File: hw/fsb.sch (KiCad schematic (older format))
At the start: 8 parts, among them J101 AMPSEAL_8_POS_VERT_WHITE_SEAL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, J102 AMPSEAL_23_POS_VERT_WHITE_SEA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

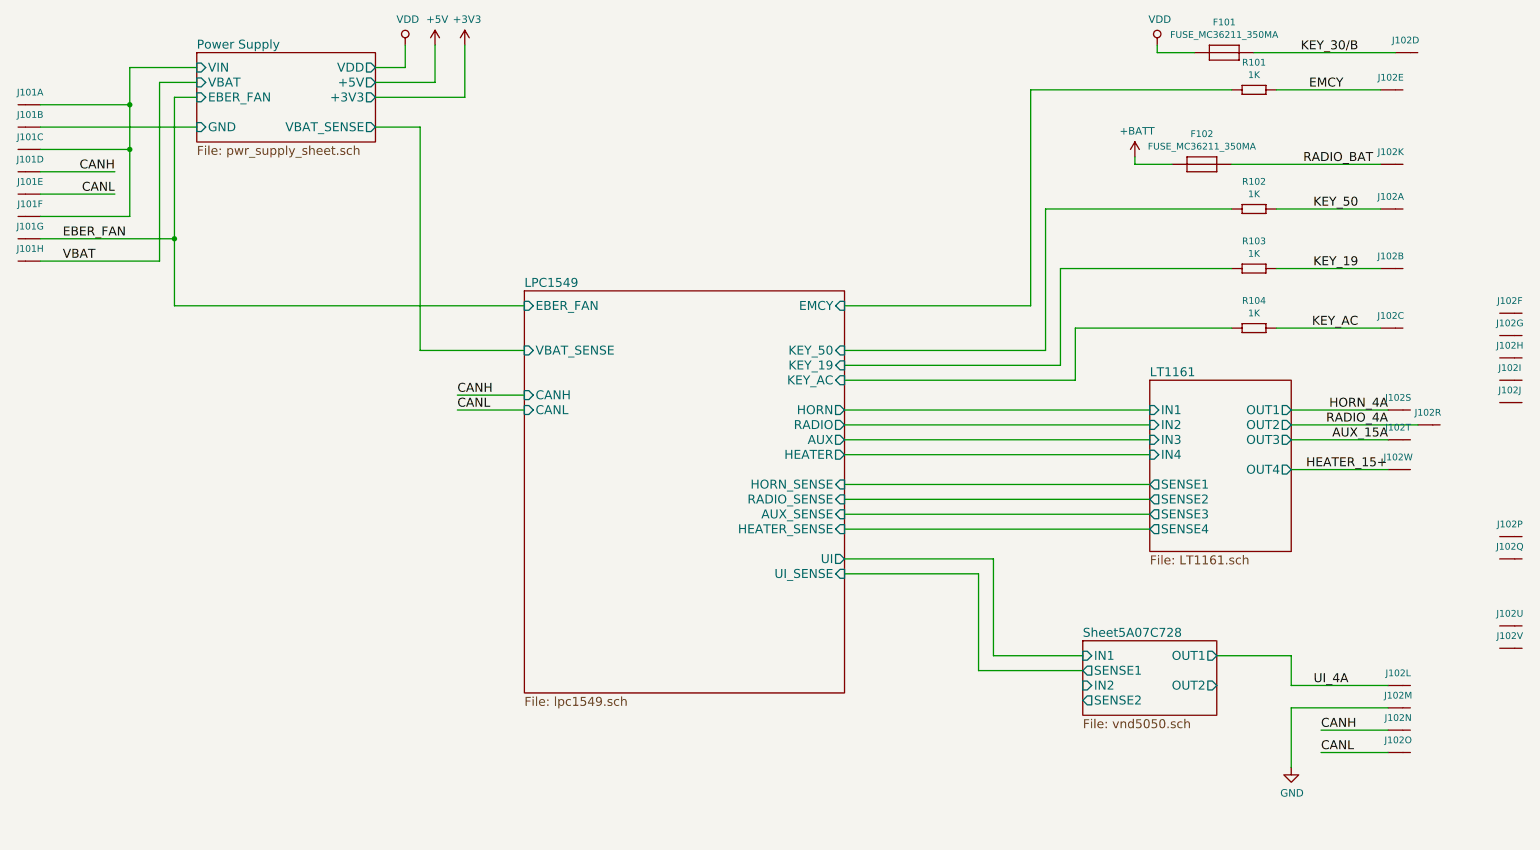
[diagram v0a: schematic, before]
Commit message: hw 2.1.0 created, not yet ordered
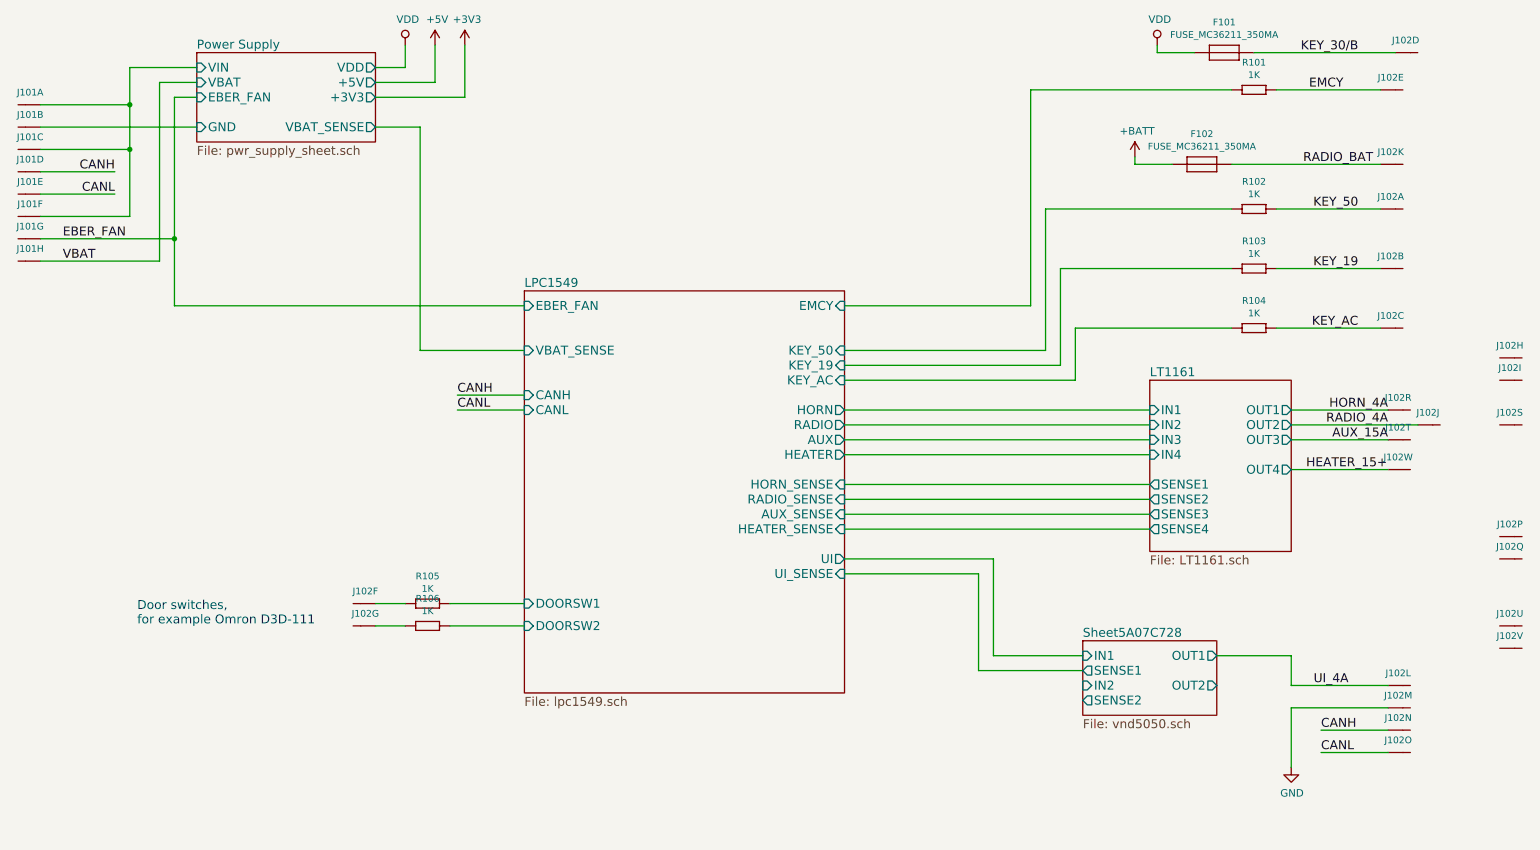
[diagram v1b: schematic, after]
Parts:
- added R105, R106: 1K, yageo:0603, symbol 1K
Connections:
- net HORN_4A: now also J102.P$18 (S); no longer J102.P$19 (S)
- net RADIO_4A: now also J102.P$10 (S); no longer J102.P$18 (S)
- net at J102.P$6 (S): now also R105.2 (R2)
- net at J102.P$7 (S): now also R106.2 (R2)
- new net LPC1549/DOORSW1: R105.1 (R1)
- new net LPC1549/DOORSW2: R106.1 (R1)
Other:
- note added: "Door switches,\nfor example Omron D3D-111"
- moved on the sheet: J102F, J102G, J102J, J102R, J102S
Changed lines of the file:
@@
 F18 "UI" O R 6400 4600 60
 F19 "UI_SENSE" I R 6400 4700 60
+F20 "DOORSW1" I L 4250 4900 60
+F21 "DOORSW2" I L 4250 5050 60
 $EndSheet
 $Comp
@@
 L AMPSEAL_23_POS_VERT_WHITE_SEALED_1-776228-2-RESCUE-fsb J102
 U 6 1 5988B296
-P 10900 2950
-F 0 "J102" H 10868 3033 45  0000 C CNN
-F 1 "AMPSEAL_23_POS_VERT_WHITE_SEALED_1-776228-2" H 10900 2950 45  0001 L BNN
-F 2 "usevolt:AMPSEAL_23_POS_776200-1" H 10930 3100 20  0001 C CNN
-F 3 "http://www.mouser.com/ds/2/418/NG_CD_776228_C13-692101.pdf" H 11000 2920 60  0001 C CNN
-F 4 "571-1-776228-2" H 11400 3320 60  0001 C CNN "1st Source Part Number"
-F 5 "1-776228-2" H 11200 3120 60  0001 C CNN "Manufacturer Part Number"
-F 6 "Mouser" H 11300 3220 60  0001 C CNN "1st Source"
-F 7 "TE Connectivity" H 11100 3020 60  0001 C CNN "Manufacturer"
-	6    10900 2950
-	1    0    0    -1
+P 3150 4900
+F 0 "J102" H 3118 4983 45  0000 C CNN
+F 1 "AMPSEAL_23_POS_VERT_WHITE_SEALED_1-776228-2" H 3150 4900 45  0001 L BNN
+F 2 "usevolt:AMPSEAL_23_POS_776200-1" H 3180 5050 20  0001 C CNN
+F 3 "http://www.mouser.com/ds/2/418/NG_CD_776228_C13-692101.pdf" H 3250 4870 60  0001 C CNN
+F 4 "571-1-776228-2" H 3650 5270 60  0001 C CNN "1st Source Part Number"
+F 5 "1-776228-2" H 3450 5070 60  0001 C CNN "Manufacturer Part Number"
+F 6 "Mouser" H 3550 5170 60  0001 C CNN "1st Source"
+F 7 "TE Connectivity" H 3350 4970 60  0001 C CNN "Manufacturer"
+	6    3150 4900
+	-1   0    0    -1
 $EndComp
 $Comp
 L AMPSEAL_23_POS_VERT_WHITE_SEALED_1-776228-2-RESCUE-fsb J102
 U 7 1 5988B310
-P 10900 3100
-F 0 "J102" H 10868 3183 45  0000 C CNN
-F 1 "AMPSEAL_23_POS_VERT_WHITE_SEALED_1-776228-2" H 10900 3100 45  0001 L BNN
-F 2 "usevolt:AMPSEAL_23_POS_776200-1" H 10930 3250 20  0001 C CNN
-F 3 "http://www.mouser.com/ds/2/418/NG_CD_776228_C13-692101.pdf" H 11000 3070 60  0001 C CNN
-F 4 "571-1-776228-2" H 11400 3470 60  0001 C CNN "1st Source Part Number"
-F 5 "1-776228-2" H 11200 3270 60  0001 C CNN "Manufacturer Part Number"
-F 6 "Mouser" H 11300 3370 60  0001 C CNN "1st Source"
-F 7 "TE Connectivity" H 11100 3170 60  0001 C CNN "Manufacturer"
-	7    10900 3100
-	1    0    0    -1
+P 3150 5050
+F 0 "J102" H 3118 5133 45  0000 C CNN
+F 1 "AMPSEAL_23_POS_VERT_WHITE_SEALED_1-776228-2" H 3150 5050 45  0001 L BNN
+F 2 "usevolt:AMPSEAL_23_POS_776200-1" H 3180 5200 20  0001 C CNN
+F 3 "http://www.mouser.com/ds/2/418/NG_CD_776228_C13-692101.pdf" H 3250 5020 60  0001 C CNN
+F 4 "571-1-776228-2" H 3650 5420 60  0001 C CNN "1st Source Part Number"
+F 5 "1-776228-2" H 3450 5220 60  0001 C CNN "Manufacturer Part Number"
+F 6 "Mouser" H 3550 5320 60  0001 C CNN "1st Source"
+F 7 "TE Connectivity" H 3350 5120 60  0001 C CNN "Manufacturer"
+	7    3150 5050
+	-1   0    0    -1
 $EndComp
 $Comp
@@
 L AMPSEAL_23_POS_VERT_WHITE_SEALED_1-776228-2-RESCUE-fsb J102
 U 10 1 5988B48A
-P 10900 3550
-F 0 "J102" H 10868 3633 45  0000 C CNN
-F 1 "AMPSEAL_23_POS_VERT_WHITE_SEALED_1-776228-2" H 10900 3550 45  0001 L BNN
-F 2 "usevolt:AMPSEAL_23_POS_776200-1" H 10930 3700 20  0001 C CNN
-F 3 "http://www.mouser.com/ds/2/418/NG_CD_776228_C13-692101.pdf" H 11000 3520 60  0001 C CNN
-F 4 "571-1-776228-2" H 11400 3920 60  0001 C CNN "1st Source Part Number"
-F 5 "1-776228-2" H 11200 3720 60  0001 C CNN "Manufacturer Part Number"
-F 6 "Mouser" H 11300 3820 60  0001 C CNN "1st Source"
-F 7 "TE Connectivity" H 11100 3620 60  0001 C CNN "Manufacturer"
-	10   10900 3550
+P 10350 3700
+F 0 "J102" H 10318 3783 45  0000 C CNN
+F 1 "AMPSEAL_23_POS_VERT_WHITE_SEALED_1-776228-2" H 10350 3700 45  0001 L BNN
+F 2 "usevolt:AMPSEAL_23_POS_776200-1" H 10380 3850 20  0001 C CNN
+F 3 "http://www.mouser.com/ds/2/418/NG_CD_776228_C13-692101.pdf" H 10450 3670 60  0001 C CNN
+F 4 "571-1-776228-2" H 10850 4070 60  0001 C CNN "1st Source Part Number"
+F 5 "1-776228-2" H 10650 3870 60  0001 C CNN "Manufacturer Part Number"
+F 6 "Mouser" H 10750 3970 60  0001 C CNN "1st Source"
+F 7 "TE Connectivity" H 10550 3770 60  0001 C CNN "Manufacturer"
+	10   10350 3700
 	1    0    0    -1
 $EndComp
@@
 L AMPSEAL_23_POS_VERT_WHITE_SEALED_1-776228-2-RESCUE-fsb J102
 U 18 1 5988B8D6
-P 10350 3700
-F 0 "J102" H 10318 3783 45  0000 C CNN
-F 1 "AMPSEAL_23_POS_VERT_WHITE_SEALED_1-776228-2" H 10350 3700 45  0001 L BNN
-F 2 "usevolt:AMPSEAL_23_POS_776200-1" H 10380 3850 20  0001 C CNN
-F 3 "http://www.mouser.com/ds/2/418/NG_CD_776228_C13-692101.pdf" H 10450 3670 60  0001 C CNN
-F 4 "571-1-776228-2" H 10850 4070 60  0001 C CNN "1st Source Part Number"
-F 5 "1-776228-2" H 10650 3870 60  0001 C CNN "Manufacturer Part Number"
-F 6 "Mouser" H 10750 3970 60  0001 C CNN "1st Source"
-F 7 "TE Connectivity" H 10550 3770 60  0001 C CNN "Manufacturer"
-	18   10350 3700
-	1    0    0    -1
-$EndComp
-$Comp
-L AMPSEAL_23_POS_VERT_WHITE_SEALED_1-776228-2-RESCUE-fsb J102
-U 19 1 5988C267
 P 10150 3600
 F 0 "J102" H 10118 3683 45  0000 C CNN
@@
 F 6 "Mouser" H 10550 3870 60  0001 C CNN "1st Source"
 F 7 "TE Connectivity" H 10350 3670 60  0001 C CNN "Manufacturer"
-	19   10150 3600
+	18   10150 3600
+	1    0    0    -1
+$EndComp
+$Comp
+L AMPSEAL_23_POS_VERT_WHITE_SEALED_1-776228-2-RESCUE-fsb J102
+U 19 1 5988C267
+P 10900 3700
+F 0 "J102" H 10868 3783 45  0000 C CNN
+F 1 "AMPSEAL_23_POS_VERT_WHITE_SEALED_1-776228-2" H 10900 3700 45  0001 L BNN
+F 2 "usevolt:AMPSEAL_23_POS_776200-1" H 10930 3850 20  0001 C CNN
+F 3 "http://www.mouser.com/ds/2/418/NG_CD_776228_C13-692101.pdf" H 11000 3670 60  0001 C CNN
+F 4 "571-1-776228-2" H 11400 4070 60  0001 C CNN "1st Source Part Number"
+F 5 "1-776228-2" H 11200 3870 60  0001 C CNN "Manufacturer Part Number"
+F 6 "Mouser" H 11300 3970 60  0001 C CNN "1st Source"
+F 7 "TE Connectivity" H 11100 3770 60  0001 C CNN "Manufacturer"
+	19   10900 3700
 	1    0    0    -1
 $EndComp
@@
 Wire Wire Line
 	7300 4700 6400 4700
+Wire Wire Line
+	4250 5050 3750 5050
+Wire Wire Line
+	3750 4900 4250 4900
+$Comp
+L 1K R105
+U 1 1 5A09BE6F
+P 3550 4900
+F 0 "R105" H 3600 5084 45  0000 C CNN
+F 1 "1K" H 3600 5000 45  0000 C CNN
+F 2 "yageo:0603" H 3580 5050 20  0001 C CNN
+F 3 "" H 3519 4939 60  0001 C CNN
+F 4 "" H 3919 5339 60  0001 C CNN "1st Source Part Number"
+F 5 "Digikey" H 3819 5239 60  0001 C CNN "1st Source"
+F 6 "RC0603FR-071KL" H 3719 5139 60  0001 C CNN "Manufacturer Part Number"
+F 7 "YAGEO" H 3619 5039 60  0001 C CNN "Manufacturer"
+	1    3550 4900
+	1    0    0    -1
+$EndComp
+$Comp
+L 1K R106
+U 1 1 5A09C192
+P 3550 5050
+F 0 "R106" H 3600 5234 45  0000 C CNN
+F 1 "1K" H 3600 5150 45  0000 C CNN
+F 2 "yageo:0603" H 3580 5200 20  0001 C CNN
+F 3 "" H 3519 5089 60  0001 C CNN
+F 4 "" H 3919 5489 60  0001 C CNN "1st Source Part Number"
+F 5 "Digikey" H 3819 5389 60  0001 C CNN "1st Source"
+F 6 "RC0603FR-071KL" H 3719 5289 60  0001 C CNN "Manufacturer Part Number"
+F 7 "YAGEO" H 3619 5189 60  0001 C CNN "Manufacturer"
+	1    3550 5050
+	1    0    0    -1
+$EndComp
+Wire Wire Line
+	3450 4900 3250 4900
+Wire Wire Line
+	3250 5050 3450 5050
+Text Notes 1650 5050 0    60   ~ 0
+Door switches,\nfor example Omron D3D-111
 $EndSCHEMATC

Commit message: making 2.2.0 pcb
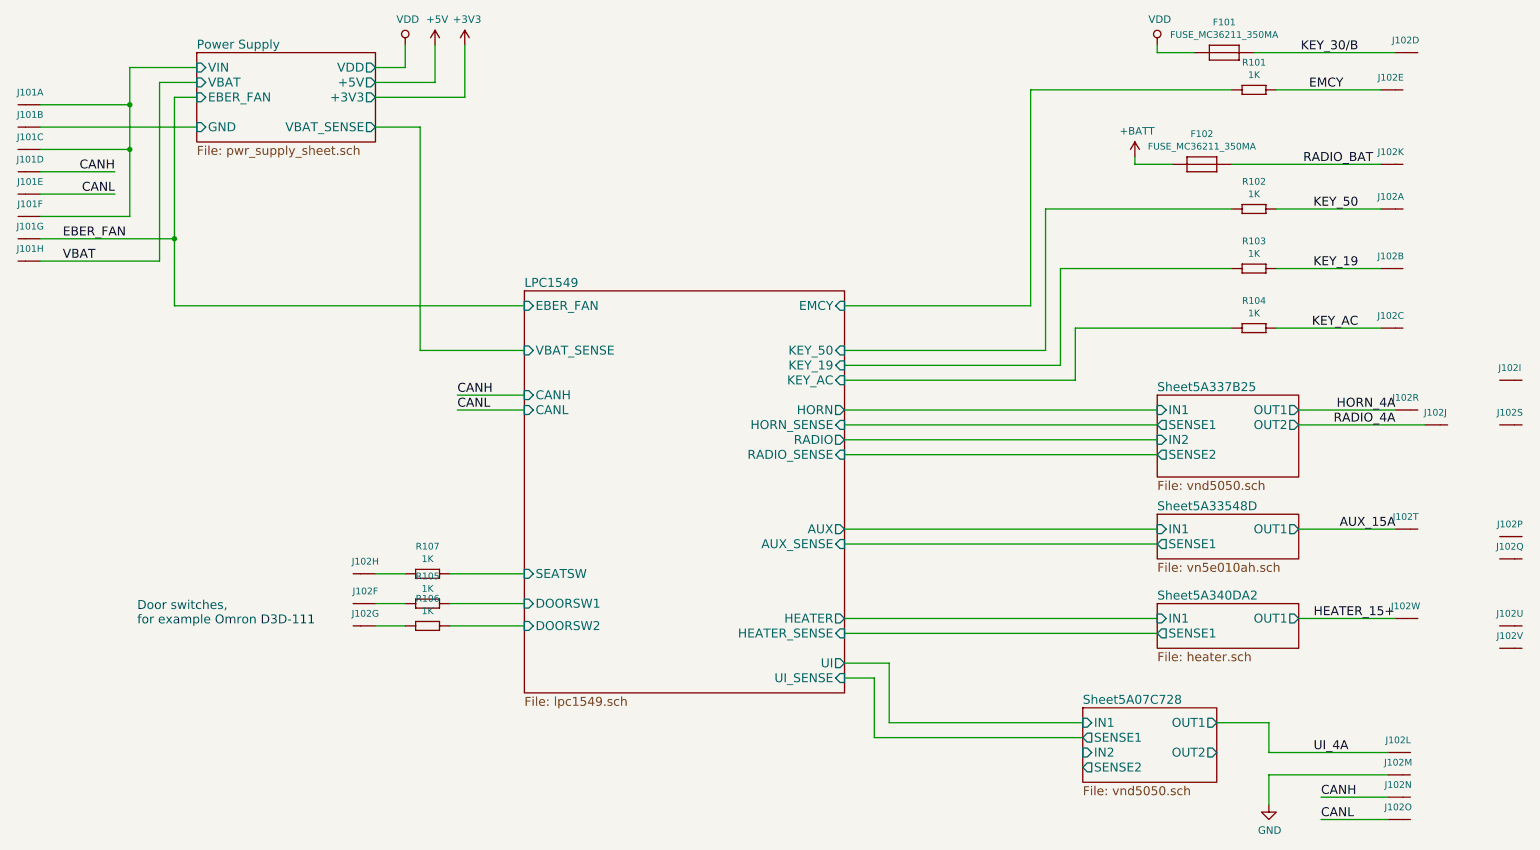
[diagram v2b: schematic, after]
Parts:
- added R107: 1K, yageo:0603, symbol 1K
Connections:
- net at J102.P$8 (S): now also R107.2 (R2)
- new net LPC1549/SEATSW: R107.1 (R1)
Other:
- moved on the sheet: J102H, J102J, J102L, J102M, J102N, J102O, J102R, J102T, J102W
